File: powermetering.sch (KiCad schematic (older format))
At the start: 182 parts, among them J1 Conn_01x04, J11 CONN_01X02, J12 CONN_01X02, J13 CONN_01X02, J14 CONN_01X02, J15 CONN_01X02, J2 Conn_01x02, J3 Conn_01x02, J4 Conn_01x02, J5 Conn_01x02, J7 CONN_01X02, J8 CONN_01X02, J9 CONN_01X02, U10 AP1117-50, U11 AP9101CK, U12 NFET, U13 NFET, U2 ADE9000, U5 ALTAIR04-900, U6 AP1117-50, U7 Si8641EB-B-IU, U8 NXE2S0505MC, U9 MCP73811T-420I-OT, Y1 Crystal

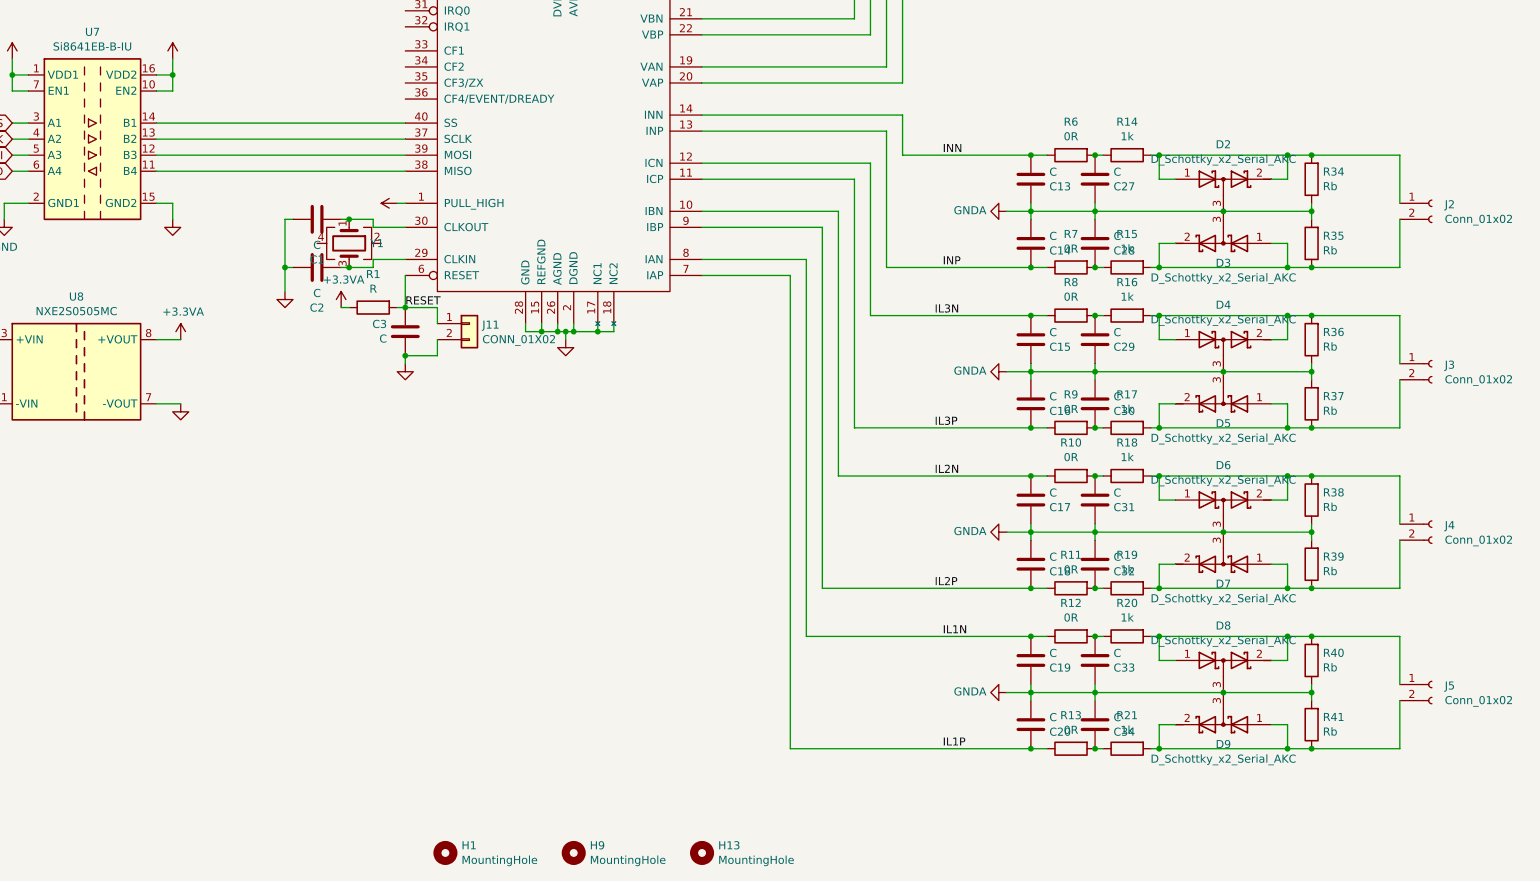
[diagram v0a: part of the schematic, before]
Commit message: small production changes
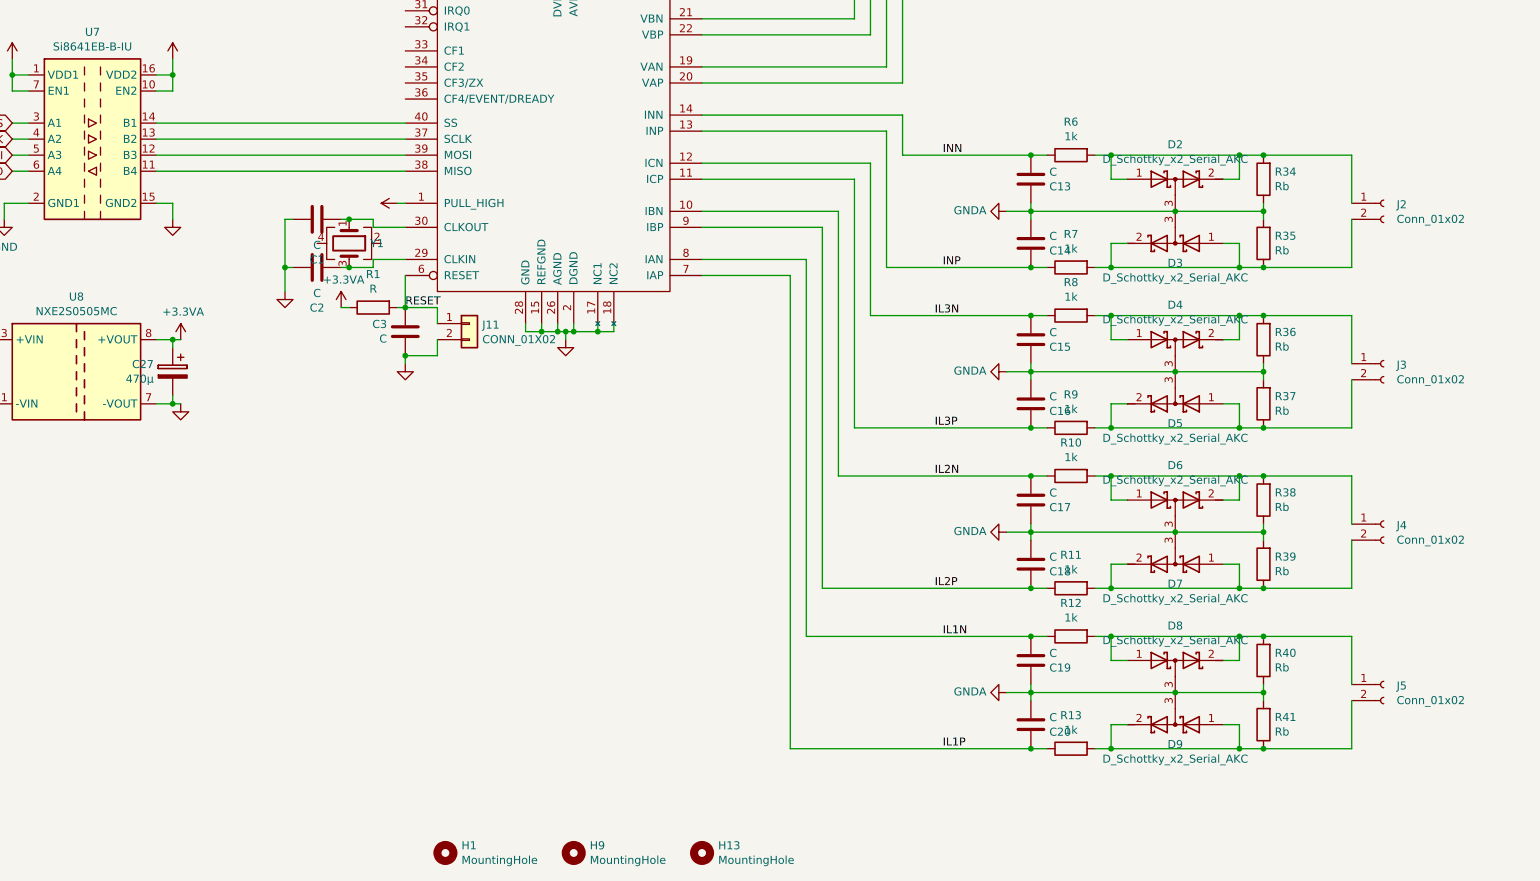
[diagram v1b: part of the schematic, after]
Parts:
- removed C27, C28, C29, C30, C31, C32, C33, C34: C, stmbl:C_0603, symbol stmbl:C
- removed R14, R15, R16, R17, R18, R19, R20, R21: 1k, stmbl:R_0603, symbol stmbl:R
- added C27: 470µ, Capacitor_SMD:CP_Elec_6.3x5.9, symbol stmbl:CP
- H1, H10, H11, H12, H13, H14, H15, H16, H2, H3, H4, H9: footprint MountingHole:MountingHole_3.2mm_M3 -> MountingHole:MountingHole_5.5mm
- J1: footprint TerminalBlock_Phoenix:TerminalBlock_Phoenix_PT-1,5-5-5.0-H_1x05_P5.00mm_Horizontal -> stmbl:RM5.08_1x5_UP
- J2, J3, J4, J5: footprint TerminalBlock_Phoenix:TerminalBlock_Phoenix_PT-1,5-2-5.0-H_1x02_P5.00mm_Horizontal -> stmbl:RM5.08_1x2_UP
- R10, R11, R12, R13, R6, R7, R8, R9: value 0R -> 1k
- R25, R26, R27, R28, R29, R30, R31, R32, R33, R42, R43, R44: footprint Resistor_SMD:R_2010_5025Metric -> stmbl:R_1206
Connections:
- net +3.3VA: now also C27.1
- net GNDA: now also C27.2
- net at D2.1 (A), D2.2 (K), J2.1 (Pin_1)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: now also R6.2
- net at D3.1 (A), D3.2 (K), J2.2 (Pin_2)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: now also R7.2
- net at D4.1 (A), D4.2 (K), J3.1 (Pin_1)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: now also R8.2
- net at D5.1 (A), D5.2 (K), J3.2 (Pin_2)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: now also R9.2
- net at D6.1 (A), D6.2 (K), J4.1 (Pin_1)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: now also R10.2
- net at D7.1 (A), D7.2 (K), J4.2 (Pin_2)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: now also R11.2
- net at D8.1 (A), D8.2 (K), J5.1 (Pin_1)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: now also R12.2
- net at D9.1 (A), D9.2 (K), J5.2 (Pin_2)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: now also R13.2
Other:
- moved on the sheet: D2, D3, D4, D5, D6, D7, D8, D9, J2, J3, J4, J5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
